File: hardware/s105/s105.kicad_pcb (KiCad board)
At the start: 2 copper layers, 86 x 159 mm, 583 parts, among them J1 Conn_01x06, P1 368255-2, Q1 BC847C, Q10 BC847C, Q11 BC847C, Q12 BC847C, Q13 BC847C, Q14 BC847C, Q15 BC847C, Q16 BC847C, Q17 BC847C, Q18 BC847C, Q19 ., Q2 BC847C, Q20 BC847C, Q21 BC847C, Q22 BC847C, Q23 BC847C, Q24 ., Q3 BC847C, Q4 ., Q5 ., Q6 BC847C, Q7 BC847C, Q8 BC847C, Q9 BC847C, U1 case only, U2 STM32F427VGT6, U3 case only, U4 case only, U5 case only, U6 LM2902, U7 SIT1042T/3, U8 case only, U9 case only, X1 8MHz 20pF, X2 NM

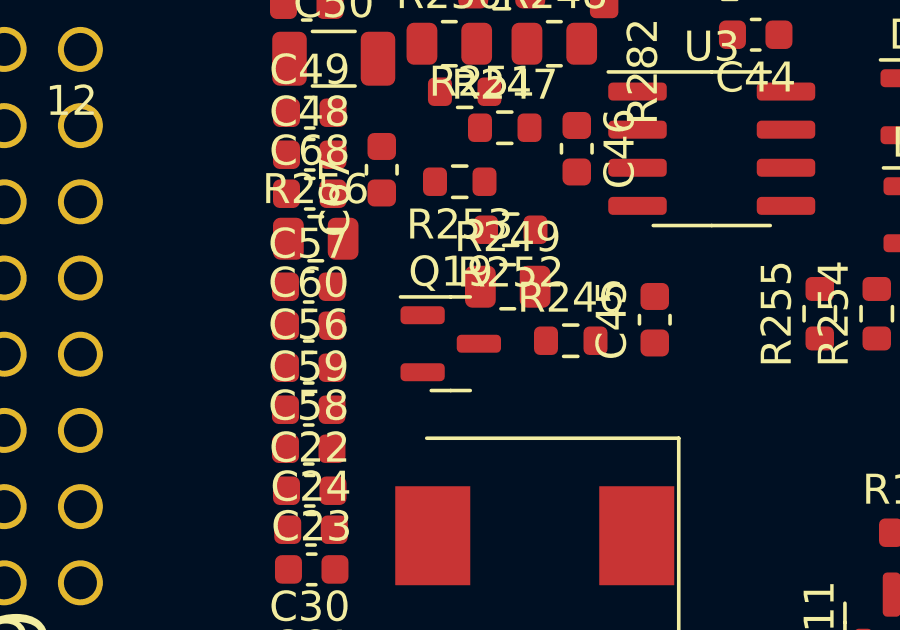
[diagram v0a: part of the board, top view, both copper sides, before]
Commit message: #4 #5 #6 #8
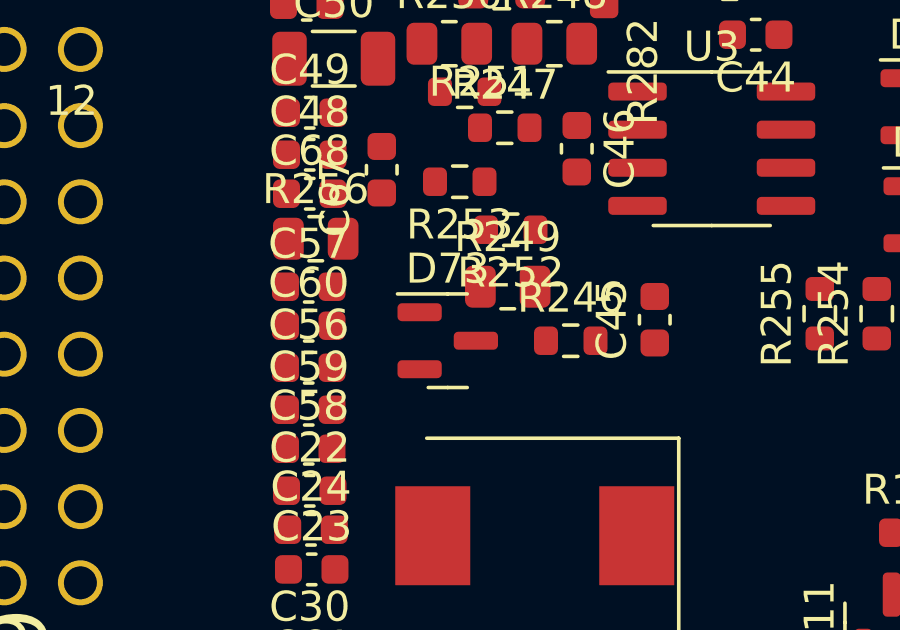
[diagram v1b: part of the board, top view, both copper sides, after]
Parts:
- removed Q19: ., Package_TO_SOT_SMD:SOT-23
- added D73: ., Package_TO_SOT_SMD:SOT-23, F.Cu at (76.1, 176.8)
- U3: value case only -> LM2903
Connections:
- R247 pad 1: Net-(R247-Pad1) -> Net-(R252-Pad2)
- R251 pad 2: Net-(R247-Pad1) -> Net-(R252-Pad2)
